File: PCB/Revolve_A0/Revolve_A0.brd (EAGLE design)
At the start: 100 x 100 mm, 409 parts, among them IC1 TMC2100-LA, IC12 TMC2100-LA, IC15 TMC2100-LA, IC2 TMC2100-LA, IC24 TMC2100-LA, IC29 LAN8710A, IC30 MTFC2GMDEA, IC31 CY7C65632, IC5 TMC2100-LA, IC6 74AHC1G126DCK, IC7 74AHC1G126DCK, Q1 AON6758, Q2 AON6758, Q3 AON6758, Q8 AON6758, U1 OSD3358-512M-BSM, U10 TPD4S012_DRY_6, U11 PCA9685PW, U19 CD4050BD, X1 22-05-7038-03, X10 22-05-7038-03, X11 22-05-7038-03, X12 22-05-7048-04, X13 22-05-7038-03, X14 22-05-7048-04, X15 22-05-7048-04, X16 22-05-7048-04, X17 22-05-7048-04, X18 22-05-7048-04, X19 22-05-7038-03, X2 MSTBA4, X20 MSTBA4, X21 MSTBA2, X22 22-05-7038-03, X24 HDMI, X25 22-05-7048-04, X26 MSTBA2, X29 22-05-7038-03, X3 MSTBA2, X4 22-05-7028-02, X5 22-05-7028-02, X6 22-05-7028-02, X7 22-05-7038-03, X8 22-05-7038-03, X9 22-05-7028-02, Y1 24MHz, Y3 25 MHz, Y4 12 MHz

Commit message: Working on the LAN layout
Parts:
- removed C106, C17, C19, C20, C22, C24, C27, C29, C31, C34, C43, C71: 0.1uF, rcl:C0402
- removed C116, C117, C118, C119, C120, C121, C122, C123, C124, C125, C126, C127, C128, C129, C130, C131: 47pF, rcl:C0402
- removed C139, C144, C145, C18, C21, C25, C36, C52, C62, C75, C76, C77, C78, C79, C81: 4.7uF, rcl:C0402
- removed C50: 10nF, rcl:C0402
- removed C90: 10uF, rcl:C0805
- removed C96: 100uF, Panasonic-EEEFK_EEEFP:RHS1V10MCN1GS
- removed IC1, IC12, IC15, IC2, IC24, IC5: TMC2100-LA, we-chip:QFN36-PAD
- removed IC31: CY7C65632, Revolve:QFN28
- removed R147: 0, DNI, rcl:R0402
- removed R148: 0, rcl:R0402
- removed R151: 10K, rcl:R0402
- removed R153: 22R, rcl:R0402
- removed R54, R86: 4.7K, rcl:R0402
- removed R91: 33, rcl:R0402
- removed U11: PCA9685PW, custom:SOP65P640X110-28N
- added C13: 0.1uF, rcl:C0402
- added C5: 18pF, rcl:C0402
- added H1, H2, H3, H4: MOUNT-HOLE3.2, holes:3,2
- added J1: (no value), OSD3358-SM-RED Platform:CTI-JTAG
- added Q9: MMBT2907, OSD3358-SM-RED Platform:SOT23-BEC
- added R143, R144: 4.7K, rcl:R0402
- added R26: 1M, rcl:R0402
- added SV3: (no value), con-lstb:MA04-2
- added SV4: (no value), con-lstb:MA03-1
- added SV5: (no value), con-lstb:MA04-1
- added U$13, U$14, U$15, U$16: TRINAMIC_TMC2130_QFN36, TMC2130-Eval_v13:TRINAMIC_QFN36
- added U2: TUSB2046BIRHBT, Texas Instruments_By_element14_Batch_1:QFN50P500X500X100-33N
- added U3, U4: TPD2E001DRSR, Texas Instruments_By_element14_Batch_1:SON95P315X315X80-7N
- added U5: SN74HC245DW, Texas Instruments_By_element14_Batch_1:SOIC127P1030X265-20N
- added U7: TLVH431, OSD3358-SM-RED Platform:SOT23-3
- added Y5: ABS07-32.768KHZ-T, OSD3358-SM-RED Platform:CRYSTAL_3.2X1.5
- C1: value 22nF -> 0.1uF
- C12, C138, C140, C141, C142: value 4.7uF -> 0.1uF
- C143: value 4.7uF -> 10uF
- C48, C80: value 10uF -> 22uF
- C6: value 0.1uF -> 18pF
- EEPROM_WP, PMIC_NRESET, SYS_5V, SYS_RTC_1V8, SYS_VDD1_3V3, SYS_VDD2_3V3, SYS_VDD3_3V3, VDDS_DDR, VDDS_PLL, VDD_CODE, VDD_MPU: value TPPAD1-13 -> TPB1,27; device testpad:P1-13 -> testpad:B1,27
- R1: value 0.1R -> 1.5K; device rcl:R0805 -> rcl:R0402
- R12: value 44.3K,1% -> 100K,1%
- R152: value 10K -> 10K,1%
- R2: value 0.1R -> 0,DNI; device rcl:R0805 -> rcl:R0402
- R22: value 10K,1% -> 13.3K,1%
- R24: value 4.7K -> 0R,DNI
- R41: value 10K -> 10K, 1%; device rcl:R0402 -> OSD3358-SM-RED Platform:R0402
- R49: value 10K -> 40.2K, 1%; device rcl:R0402 -> OSD3358-SM-RED Platform:R0402
- R53: value 2.2R -> 499; device rcl:R0402 -> OSD3358-SM-RED Platform:R0402
- R87: value 650R, 1% -> 4.7K
- SV2: device con-lstb:MA05-1 -> con-lstb:MA04-2
- U$9: value SN74AUC1G74DCTR -> TRINAMIC_TMC2130_QFN36; device Revolve:S-PDSO-G8 -> TMC2130-Eval_v13:TRINAMIC_QFN36
- Y1: value 24MHz -> 25MHz
- Y4: value 12 MHz -> 6 MHz
- moved PMIC_NRESET 474.8 mm to (44.7, 69.9), flipped to the bottom
- moved VDDS_PLL 452.8 mm to (38.5, 70.0), flipped to the bottom
- moved VDD_MPU 431.2 mm to (37.0, 70.0), flipped to the bottom
- moved VDD_CODE 397.7 mm to (38.8, 57.7), flipped to the bottom
- moved VDDS_DDR 376.0 mm to (37.3, 57.7), flipped to the bottom
- moved SV2 333.6 mm to (38.2, 33.5)
- moved EEPROM_WP 319.6 mm to (46.5, 51.6)
- moved R141 276.1 mm to (16.3, 23.8)
- moved R140 272.5 mm to (16.3, 24.9), turned to 180 degrees
- moved R138 255.3 mm to (20.8, 27.9), turned to 270 degrees
- moved R139 250.0 mm to (20.8, 16.6), turned to 90 degrees
- moved C88 240.6 mm to (16.3, 19.1), turned to 180 degrees
- moved C99 234.2 mm to (17.4, 17.2), turned to 270 degrees
- moved R126 232.9 mm to (16.3, 21.5)
- moved C87 232.5 mm to (16.3, 20.4), turned to 180 degrees
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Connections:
- net N$1 renamed PMIC_PWR_EN
- net N$103 renamed PMIC_SCL
- net N$104 renamed PMIC_SDA
- net N$121 renamed PMIC_LDO_PGOOD
- net N$143 renamed PMIC_NWAKEUP
- net N$144 renamed PMIC_NINT
- net N$157 renamed TXP
- net N$158 renamed TXN
- net N$159 renamed RXP
- net N$160 renamed RXN
- net N$174 renamed EEPROM_WP
- net VBUS renamed USB_HOST_5V
- removed net 12MHZ: R91.1, U$7.27
- removed net D+: U$8.P$3, U10.1
- removed net D-: U$8.P$2, U10.2
- removed net ENABLE_A: IC24.22
- removed net ENABLE_E: IC12.22
- removed net ENABLE_H: IC15.22
- removed net ENABLE_X: IC1.22, U$2.22
- removed net ENABLE_Y: IC2.22
- removed net ENABLE_Z: IC5.22
- removed net END_STOP_X_1: U19.2
- removed net END_STOP_X_2: U19.10
- removed net END_STOP_Y_1: U19.4
- removed net END_STOP_Y_2: U19.12
- removed net END_STOP_Z_1: U19.6
- removed net END_STOP_Z_2: U19.15
- removed net FAULT_X0: U$2.20
- removed net FAULT_X1: U$2.21
- removed net I2C2_SCL: U11.26
- removed net I2C2_SDA: U11.27
- removed net ID: U$8.P$4, U10.3
- removed net IREF_A_RAW: R73.2, U11.8
- removed net IREF_E_RAW: R60.2, U11.21
- removed net IREF_H1: C81.1, R43.2, R73.1
- removed net IREF_H_RAW: R31.2, U11.22
- removed net IREF_X1: C145.1, R140.2, R141.1
- removed net IREF_X_RAW: R141.2, R41.2, U11.18
- removed net IREF_Y_RAW: R37.2, U11.19
- removed net IREF_Z_RAW: R58.2, U11.20
- removed net N$100: IC15.5
- removed net N$101: IC15.18
- removed net N$102: IC15.19
- removed net N$105: SYS_VDD1_3V3.TP, U1.F6, U1.F7, U1.G6, U1.G7
- removed net N$107: C70.1, IC15.26, R52.2
- removed net N$108: C71.1, IC1.26, R53.2
- removed net N$110: C72.1, IC2.26, R59.2
- removed net N$111: C74.1, IC12.26, R71.2
- removed net N$112: IC12.32, X17.1
- removed net N$119: IC15.32, X18.1
- removed net N$120: SYS_VDD3_3V3.TP, U1.F8, U1.G8, U1.H7, U1.H8, U1.J7, U1.J8, U1.K8, U1.L8
- removed net N$131: C52.1, IC24.23, R43.1
- removed net N$133: IC24.3
- removed net N$135: IC24.34, X25.2
- removed net N$136: C55.2, IC24.25, R72.1
- removed net N$138: IC24.4
- removed net N$139: IC24.5
- removed net N$140: IC24.18
- removed net N$141: IC24.19
- removed net N$142: SYS_RTC_1V8.TP, U1.K11, U1.L11
- removed net N$146: U1.F9, U1.G9, U1.H9, U1.J9, U1.K9, U1.L9
- removed net N$148: IC24.32, X25.1
- removed net N$165: U1.T7
- removed net N$166: C86.2, R126.1, U$2.25
- removed net N$175: R86.2
- removed net N$178: U1.T16
- removed net N$18: IC1.14, R1.2
- removed net N$185: C144.1, R140.1, U$2.23
- removed net N$186: U1.T12
- removed net N$187: C155.1, IC31.27, R147.1, R148.1
- removed net N$188: U1.R12
- removed net N$190: U1.T13
- removed net N$191: IC31.14, IC31.21, IC31.28, IC31.5, IC31.9
- removed net N$197: IC31.13, U$6.3
- removed net N$198: IC31.12, U$6.2
- removed net N$199: IC31.16, U$6.7
- removed net N$200: IC31.15, U$6.6
- removed net N$202: U$9.2, U$9.3
- removed net N$205: R91.2, U$9.5
- removed net N$210: SV2.5, U1.B12
- removed net N$213: C157.2, IC31.11, Y4.P$1
- removed net N$215: SV2.4, U1.A12
- removed net N$26: C25.1, IC5.23, R27.1
- removed net N$31: C21.2, IC1.25, R53.1
- removed net N$47: C33.2, IC2.25, R59.1
- removed net N$50: IC5.34, X16.2
- removed net N$51: C37.2, IC5.25, R70.1
- removed net N$53: IC2.5
- removed net N$54: IC5.4
- removed net N$55: IC5.5
- removed net N$56: IC2.18
- removed net N$57: IC5.18
- removed net N$58: IC5.19
- removed net N$60: C50.2, L1.P$2, U$10.2
- removed net N$65: IC2.19
- removed net N$73: C50.1, U$10.6
- removed net N$74: C62.1, IC12.23, R35.1
- removed net N$76: IC12.3
- removed net N$78: IC12.34, X17.2
- removed net N$79: C65.2, IC12.25, R71.1
- removed net N$81: IC12.4
- removed net N$82: IC12.5
- removed net N$83: IC12.18
- removed net N$84: IC12.19
- removed net N$89: C36.1, IC15.23, R50.1
- removed net N$91: IC15.3
- removed net N$94: IC15.34, X18.2
- removed net N$95: C68.2, IC15.25, R52.1
- removed net N$99: IC15.4
- removed net SPI0_CS0: U1.A14
- removed net SPI0_CS1: U1.C14
- removed net USB1_OCN: U1.R15
- removed net XDMA_EVENT_INTR0: U$9.1, U1.A4
- removed net X_CFG1: IC1.4
- removed net X_CFG2: IC1.3
- new net 5VIN_Y: C72.1, R59.2, U$13.26
- new net 5VOUT_A: C55.2, R72.1, R73.2, U$16.25
- new net 5VOUT_E: C65.2, R35.2, R71.1, U$14.25
- new net 5VOUT_H: C68.2, R31.2, R52.1, U$15.25
- new net 5VOUT_X: C86.2, R126.1, R140.2, U$2.25
- new net 5VOUT_Y: C33.2, R37.2, R59.1, U$13.25
- new net 5VOUT_Z: C37.2, R27.2, R70.1, U$9.25
- new net CLKOUT1_25MHZ: R2.1, U1.A4
- new net CLKOUT2_48MHZ: U1.B4, U2.27
- new net ECAP1: SV5.3, U1.B12
- new net ECAP2: SV5.2, U1.A12
- new net EHRPWM1A: U1.P12, U5.6
- new net EHRPWM1B: U1.T13, U5.7
- new net EHRPWM2A: U1.T4, U5.8
- new net EHRPWM2B: U1.P5, U5.9
- new net EMU0: J1.13, U1.E2
- new net EMU1: J1.14, U1.E3
- new net ENABLE_B: SV2.4
- new net ENABLE_C: SV3.3
- new net END_STOP_X1: U1.N14, U19.2
- new net END_STOP_X2: U1.R12, U19.10
- new net END_STOP_Y1: U1.T16, U19.4
- new net END_STOP_Y2: U1.P3, U19.12
- new net END_STOP_Z1: U1.T6, U19.6
- new net END_STOP_Z2: U1.P7, U19.15
- new net FAULT_A: R44.1, U$16.20, U$16.21
- new net FAULT_B: SV2.2
- new net FAULT_C: SV3.1
- new net GPIO0_18: U1.J15
- new net GPIO0_26: U1.R5
- new net I2C1_SCL: U1.B11
- new net I2C1_SDA: U1.A11
- new net N$1: R41.1, R49.2, U7.1
- new net N$25: R152.1, U1.M16
- new net QUAD_ENCODER_A: U1.R13
- new net QUAD_ENCODER_B: U1.P13
- new net SPI0_CSA: U$16.2, U1.J14
- new net SPI0_CSE: U$14.2, U1.T12
- new net SPI0_CSH: U$15.2, U1.R7
- new net SPI0_CSY: U$13.2, U1.C14
- new net SPI0_CSZ: U$9.2, U1.T7
- new net SPI1_CS0: SV3.4, U1.B10
- new net SPI1_CS1: SV2.3, U1.A10
- new net SPI1_MISO: SV2.6, SV3.6, U1.C12
- new net SPI1_MOSI: SV2.8, SV3.8, U1.C13
- new net SPI1_SCLK: SV2.1, SV3.2, U1.C5
- new net SW: C2.1, L1.P$2, U$10.2
- new net SYS_RTC_1V8: Q9.C, R49.1, SYS_RTC_1V8.TP, U1.K11, U1.L11, U7.3
- new net SYS_VDD1_3V3: C13.1, C140.1, C141.1, C142.1, C143.1, C150.1, C155.1, IC29.12, IC30.C6, IC30.E6, IC30.F5, IC30.J10, IC30.K9, IC30.M4, IC30.N4, IC30.P3, IC30.P5, L2.1, R1.2, R127.2, R128.2, R129.2, R130.2, R131.2, R132.2, R133.2, R134.2, R135.2, R136.2, R137.2, R24.1, R85.1, R88.2, SYS_VDD1_3V3.TP, U1.F6, U1.F7, U1.G6, U1.G7, U2.25, U2.26, U2.3
- new net SYS_VDD3_3V3: Q9.E, R41.2, R53.2, SYS_VDD3_3V3.TP, U1.F8, U1.F9, U1.G8, U1.G9, U1.H7, U1.H8, U1.H9, U1.J7, U1.J8, U1.J9, U1.K8, U1.K9, U1.L8, U1.L9
- new net TCK: J1.11, U1.D1
- new net TDI: J1.3, U1.C1
- new net TDO: J1.7, U1.C2
- new net TIMER4: U1.M1, U5.2
- new net TIMER5: U1.N3, U5.3
- new net TIMER6: U1.N2, U5.4
- new net TIMER7: U1.N1, U5.5
- new net TK_A: U1.D7
- new net TK_E: U1.C7
- new net TK_H: U1.C8
- new net TK_HBP: U1.C9
- new net TMS: J1.1, U1.D2
- new net TRSRTN: J1.2
- new net TRSTN: U1.D3
- new net UART4_RXD: SV4.1, U1.P15
- new net UART4_TXD: SV4.2, U1.R16
- new net USB1_DM3: U$6.2, U2.19, U4.3
- new net USB1_DM4: U$6.6, U2.23, U3.3
- new net USB1_DP3: U$6.3, U2.20, U4.6
- new net USB1_DP4: U$6.7, U2.24, U3.6
- new net USB_XTAL1: C157.2, U2.30, Y4.P$1
- new net VCC: U3.1, U4.1
- new net VCC_E: C74.1, R71.2, U$14.26
- new net VCC_H: C70.1, R52.2, U$15.26
- net +24V: now also C1.2, U$13.16, U$13.30, U$13.31, U$14.16, U$14.30, U$14.31, U$15.16, U$15.30, U$15.31, U$16.16, U$16.30, U$16.31, U$9.16, U$9.30, U$9.31; no longer C19.1, C20.2, C22.2, C24.1, C27.1, C29.1, C31.1, C34.1, C43.1, C6.1, C90.1, C96.+, IC1.16, IC1.30, IC1.31, IC12.16, IC12.30, IC12.31, IC15.16, IC15.30, IC15.31, IC2.16, IC2.30, IC2.31, IC24.16, IC24.30, IC24.31, IC5.16, IC5.30, IC5.31
- net +3V3: now also R143.1, R144.1, U$13.8, U$14.8, U$15.8, U$16.8; no longer C106.1, C2.1, IC1.8, IC12.8, IC15.8, IC2.8, IC24.8, IC5.8, R24.2, R54.2, U$9.6, U$9.7
- net +5V: no longer R147.2
- net CGND: now also U$3.SHD1, U$3.SHD2, U$5.A10, U$5.A11, U$5.A12, U$5.A9, U$6.A10, U$6.A11, U$6.A12, U$6.A9, U$8.P$10, U$8.P$11, U$8.P$6, U$8.P$7, U$8.P$8, U$8.P$9, X24.PAD1, X24.PAD2, X24.PAD3, X24.PAD4
- net DIR_A: now also U$16.7; no longer IC24.7
- net DIR_B: now also SV2.5
- net DIR_C: now also SV3.5
- net DIR_E: now also U$14.7; no longer IC12.7
- net DIR_H: now also U$15.7; no longer IC15.7
- net DIR_X: no longer IC1.7
- net DIR_Y: now also U$13.7; no longer IC2.7
- net DIR_Z: now also U$9.7; no longer IC5.7
- net EMMC_RST: no longer U1.R13
- net ENABLE: now also U5.19; no longer U11.23
- net FAN0: now also U5.14; no longer U11.13
- net FAN1: now also U5.13; no longer U11.15
- net FAN2: now also U5.12; no longer U11.16
- net FAN3: now also U5.11; no longer U11.17
- net FAULT_E: now also U$14.20, U$14.21; no longer IC12.20
- net FAULT_H: now also U$15.20, U$15.21; no longer IC15.20, IC24.20, R44.1
- net FAULT_X: now also R143.2, U$2.20, U$2.21, U1.T5; no longer IC1.20, R54.1
- net FAULT_Y: now also R144.2, U$13.20, U$13.21; no longer IC2.20, R24.1
- net FAULT_Z: now also U$9.20, U$9.21; no longer IC5.20
- net GND: now also C1.1, C13.2, J1.10, J1.12, J1.16, J1.20, J1.8, R141.1, R152.2, R43.1, R50.1, R58.1, R6.1, R60.1, SV4.3, SV5.1, U$13.1, U$13.11, U$13.12, U$13.17, U$13.22, U$13.24, U$13.35, U$13.36, U$13.9, U$13.GND_PAD, U$14.1, U$14.11, U$14.12, U$14.17, U$14.22, U$14.24, U$14.35, U$14.36, U$14.9, U$14.GND_PAD, U$15.1, U$15.11, U$15.12, U$15.17, U$15.22, U$15.24, U$15.35, U$15.36, U$15.9, U$15.GND_PAD, U$16.1, U$16.11, U$16.12, U$16.17, U$16.22, U$16.24, U$16.35, U$16.36, U$16.9, U$16.GND_PAD, U$2.22, U$2.9, U$9.1, U$9.11, U$9.12, U$9.17, U$9.22, U$9.24, U$9.35, U$9.36, U$9.9, U$9.GND_PAD, U2.28, U2.7, U2.8, U5.10; no longer C106.2, C116.2, C117.2, C118.2, C119.2, C120.2, C121.2, C122.2, C123.2, C124.2, C125.2, C126.2, C127.2, C128.2, C129.2, C130.2, C131.2, C139.2, C144.2, C145.2, C17.2, C18.2, C19.2, C2.2, C20.1, C21.1, C24.2, C25.2, C27.2, C29.2, C31.2, C34.2, C36.2, C43.2, C52.2, C6.2, C62.2, C71.2, C75.2, C76.2, C77.2, C78.2, C79.2, C81.2, C90.2, C96.-, IC1.1, IC1.10, IC1.11, IC1.12, IC1.24, IC1.35, IC1.36, IC1.TP, IC12.1, IC12.10, IC12.11, IC12.12, IC12.24, IC12.35, IC12.36, IC12.TP, IC15.1, IC15.10, IC15.11, IC15.12, IC15.24, IC15.35, IC15.36, IC15.TP, IC2.1, IC2.10, IC2.11, IC2.12, IC2.24, IC2.35, IC2.36, IC2.TP, IC24.1, IC24.10, IC24.11, IC24.12, IC24.24, IC24.35, IC24.36, IC24.TP, IC31.29, IC5.1, IC5.10, IC5.11, IC5.12, IC5.24, IC5.35, IC5.36, IC5.TP, R1.1, R151.1, R2.1, R86.1, SV2.1, U$5.A10, U$5.A11, U$5.A12, U$5.A9, U$6.A10, U$6.A11, U$6.A12, U$6.A9, U$8.P$10, U$8.P$11, U$8.P$6, U$8.P$7, U$8.P$8, U$8.P$9, U$9.4, U11.14
- net HDMI_1V8: now also C12.1
- net HDMI_INT: now also U1.R15; no longer U1.T15
- net HEATER_A: now also U5.15; no longer U11.12
- net HEATER_E: now also U5.18; no longer U1.P12
- net HEATER_H: now also U5.17; no longer U11.9
- net HEATER_HBP: now also U5.16; no longer U11.10
- net IREF_E: now also R35.1, R60.2, U$14.23; no longer C79.1, R35.2, R60.1
- net IREF_H: now also U$15.23; no longer C75.1
- net IREF_X: now also R140.1, R141.2, U$2.23; no longer C77.1, R41.1, R49.2
- net IREF_Y: now also U$13.23; no longer C76.1
- net IREF_Z: now also R27.1, R58.2, U$9.23; no longer C78.1, R27.2, R58.1
- net LCD_D0: no longer C116.1
- net LCD_D1: no longer C117.1
- net LCD_D10: no longer C126.1
- net LCD_D11: no longer C127.1
- net LCD_D12: no longer C128.1
- net LCD_D13: no longer C129.1
- net LCD_D14: no longer C130.1
- net LCD_D15: no longer C131.1
- net LCD_D2: no longer C118.1
- net LCD_D3: no longer C119.1
- net LCD_D4: no longer C120.1
- net LCD_D5: no longer C121.1
- net LCD_D6: no longer C122.1
- net LCD_D7: no longer C123.1
- net LCD_D8: no longer C124.1
- net LCD_D9: no longer C125.1
- net LCD_DE: no longer R153.2
- net LCD_PCLK: no longer R153.1
- net N$109: now also U$9.26; no longer IC5.26
- net N$113: now also U$15.13; no longer IC15.13
- net N$12: now also U$15.27; no longer IC15.27
- net N$126: now also U$16.14; no longer IC24.14
- net N$128: now also U$16.33; no longer IC24.33
- net N$13: now also U$15.14; no longer IC15.14
- net N$132: now also U$16.28; no longer IC24.28
- net N$134: now also U$16.15; no longer IC24.15
- net N$137: now also U$16.29; no longer IC24.29
- net N$14: now also U$9.27; no longer IC5.27
- net N$145: now also U$16.26; no longer IC24.26
- net N$147: now also U$16.13; no longer IC24.13
- net N$15: now also U$9.14; no longer IC5.14
- net N$16: now also U$9.32, X16.2; no longer C1.1, IC1.28
- net N$17: now also U2.10, U2.14, U2.18, U2.22; no longer C1.2, IC1.27
- net N$180: now also R2.2
- net N$19: now also U$13.32, X15.2; no longer IC1.33, R2.2
- net N$192: now also R24.2, U2.31; no longer IC31.8
- net N$193: now also U2.12; no longer IC31.4
- net N$194: now also U2.11; no longer IC31.3
- net N$195: now also U2.16; no longer IC31.7
- net N$196: now also U2.15; no longer IC31.6
- net N$2: now also U$13.13; no longer IC2.13
- net N$20: now also U$13.34, X15.1; no longer C12.1, IC1.23, R49.1
- net N$214: now also U2.29; no longer IC31.10
- net N$22: now also U$14.34, X17.1; no longer IC2.32, X15.1
- net N$24: now also U$9.33; no longer IC5.33
- net N$27: now also U$9.28; no longer IC5.28
- net N$28: now also U$14.32, X17.2; no longer IC5.3
- net N$29: now also U$9.15; no longer IC5.15
- net N$3: now also U$13.27; no longer IC2.27
- net N$30: now also U$15.33; no longer IC15.33
- net N$32: now also U$15.34, X18.1; no longer IC5.32, X16.1
- net N$33: now also C5.1, C6.1, U1.B5; no longer C22.1, IC1.29
- net N$35: now also U$13.14; no longer IC2.14
- net N$36: now also U$13.33; no longer IC2.33
- net N$37: now also U$9.13; no longer IC5.13
- net N$38: now also U$15.32, X18.2; no longer C18.1, IC2.23, R6.1
- net N$39: now also U$14.13; no longer IC12.13
- net N$4: now also Q9.B, R53.1, U7.2; no longer SV2.3, U1.C12
- net N$41: now also U$13.28; no longer IC2.28
- net N$42: now also C6.2, R26.2, U1.A5, Y5.P$2; no longer IC2.3
- net N$43: now also C5.2, R26.1, U1.A6, Y5.P$1; no longer IC1.19
- net N$44: now also U$16.34, X25.1; no longer IC1.5
- net N$45: now also U$13.15; no longer IC2.15
- net N$46: now also U$16.32, X25.2; no longer IC2.34, X15.2
- net N$48: now also U$13.29; no longer IC2.29
- net N$49: now also R43.2, R73.1, U$16.23; no longer IC2.4
- net N$5: now also C2.2, U$10.6; no longer SV2.2, U1.C13
- net N$52: now also U$9.29; no longer IC5.29
- net N$6: now also U$9.34, X16.1; no longer IC1.18
- net N$70: now also U$14.27; no longer IC12.27
- net N$71: now also U$14.14; no longer IC12.14
- net N$72: now also U$14.33; no longer IC12.33
- net N$75: now also U$14.28; no longer IC12.28
- net N$77: now also U$14.15; no longer IC12.15
- net N$80: now also U$14.29; no longer IC12.29
- net N$90: now also U$15.28; no longer IC15.28
- net N$92: now also U$15.15; no longer IC15.15
- net N$96: now also U$16.27; no longer IC24.27
- net N$98: now also U$15.29; no longer IC15.29
- net SPI0_CSX: now also U1.A14
- net SPI0_MISO: now also U$13.5, U$14.5, U$15.5, U$16.5, U$9.5
- net SPI0_MOSI: now also U$13.4, U$14.4, U$15.4, U$16.4, U$9.4
- net SPI0_SCLK: now also U$13.3, U$14.3, U$15.3, U$16.3, U$9.3
- net STEP_A: now also U$16.6; no longer IC24.6
- net STEP_B: now also SV2.7
- net STEP_C: now also SV3.7
- net STEP_E: now also U$14.6; no longer IC12.6
- net STEP_H: now also U$15.6; no longer IC15.6
- net STEP_X: no longer IC1.6
- net STEP_Y: now also U$13.6; no longer IC2.6
- net STEP_Z: now also U$9.6; no longer IC5.6
- net SYS_5V: now also U5.1, U5.20; no longer C17.1, R148.2, R88.2, U11.1, U11.2, U11.24, U11.28, U11.3, U11.4, U11.5
- net SYS_RESETN: now also U1.N12, U1.P11, U1.R11
- net SYS_VDD2_3V3: now also SV5.4
- net USB0_DM: now also U$8.P$2, U10.2
- net USB0_DP: now also U$8.P$3, U10.1
- net USB0_ID: now also U$8.P$4, U10.3
- net USB1_DM: now also U2.2; no longer IC31.1
- net USB1_DP: now also R1.1, U2.1; no longer IC31.2
- net USB_DC: no longer IC31.22, R151.2
- net USB_RESET: now also U2.4; no longer IC31.17
- net USR0: now also U1.T15; no longer U1.P13
- net VDD_3V3B: no longer C139.1, C140.1, C141.1, C142.1, C143.1, C150.1, IC29.12, IC30.C6, IC30.E6, IC30.F5, IC30.J10, IC30.K9, IC30.M4, IC30.N4, IC30.P3, IC30.P5, L2.1, R127.2, R128.2, R129.2, R130.2, R131.2, R132.2, R133.2, R134.2, R135.2, R136.2, R137.2, R85.1
- net X_A1: now also X14.1; no longer X14.2
- net X_A2: now also X14.2; no longer X14.1
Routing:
- net SPI0_MISO: track 0.00 -> 164.0 mm, vias 0 -> 7
- net FAN3: track 148.3 -> 0.00 mm, vias 2 -> 0
- net FAN2: track 141.6 -> 0.00 mm, vias 2 -> 0
- net FAN1: track 136.2 -> 0.00 mm, vias 2 -> 0
- net FAN0: track 135.4 -> 0.00 mm, vias 4 -> 0
- net SYS_RESETN: track 12.6 -> 141.1 mm, vias 0 -> 5
- net SPI0_MOSI: track 0.00 -> 125.8 mm, vias 0 -> 6
- net SPI0_SCLK: track 0.00 -> 121.9 mm, vias 0 -> 6
- net IREF_A_RAW: track 113.0 -> 0.00 mm, vias 4 -> 0
- net SYS_5V: track 94.9 -> 0.64 mm, vias 4 -> 1
- net IREF_H_RAW: track 82.0 -> 0.00 mm, vias 2 -> 0
- net N$125: track 1.12 -> 76.7 mm, vias 0 -> 2
- net N$124: track 1.18 -> 75.7 mm, vias 0 -> 2
- net N$123: track 1.18 -> 74.7 mm, vias 0 -> 2
- net N$201: track 0.00 -> 73.0 mm, vias 0 -> 2
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- added copper zone on layer 1, net +5V
- added copper zone on layer 3, net N$18
- added copper zone on layer 1, net SW
- added copper zone on layer 3, net SW
- added copper zone on layer 1, net SYS_5V
- added copper zone on layer 1, net SYS_RTC_1V8
- added copper zone on layer 1, net SYS_VDD1_3V3
- added copper zone on layer 3, net SYS_VDD1_3V3
- added copper zone on layer 1, net SYS_VDD2_3V3
- added copper zone on layer 1, net SYS_VDD3_3V3
- added copper zone on layer 1, net SYS_VDD_1V8
- added copper zone on layer 1, net USB_DC
- added copper zone on layer 1, net VIN_BAT
- removed copper zone on layer 3, net VDD_3V3B
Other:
- outline, holes or cut-outs redrawn

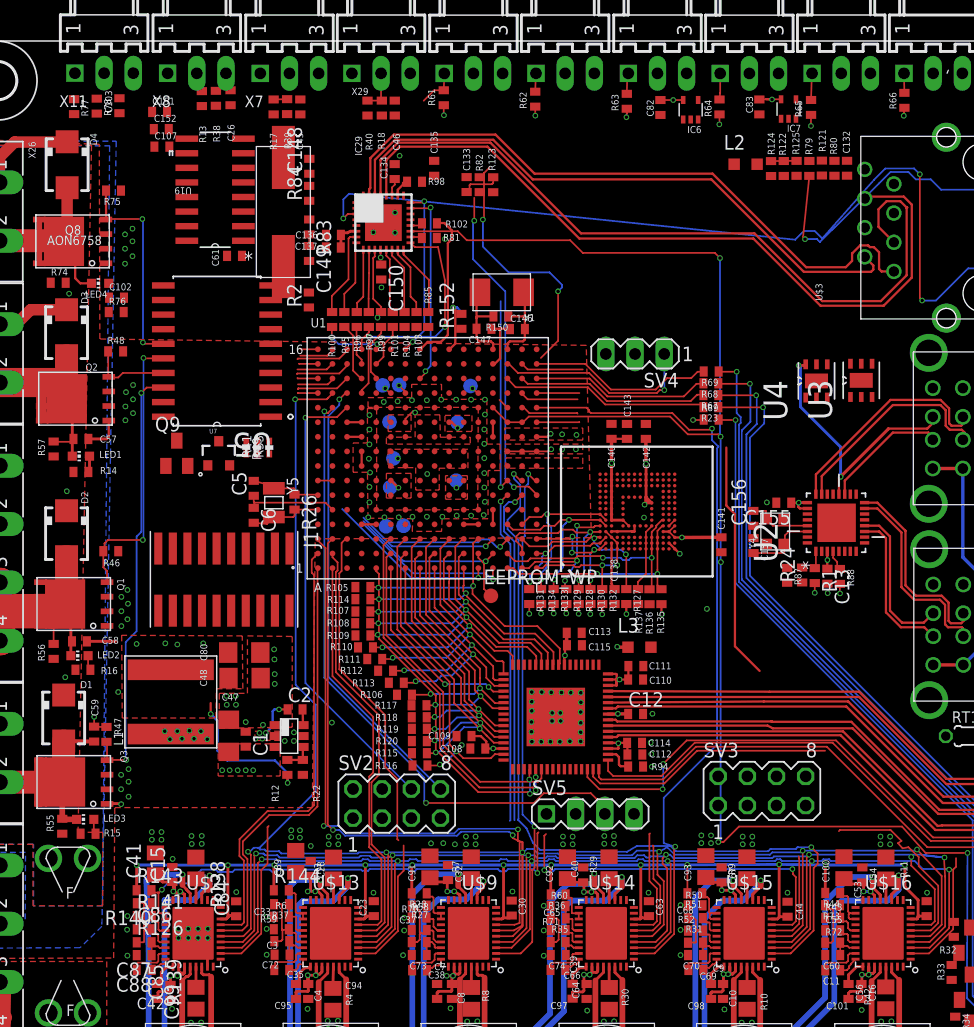
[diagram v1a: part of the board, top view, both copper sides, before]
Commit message: Working on layout
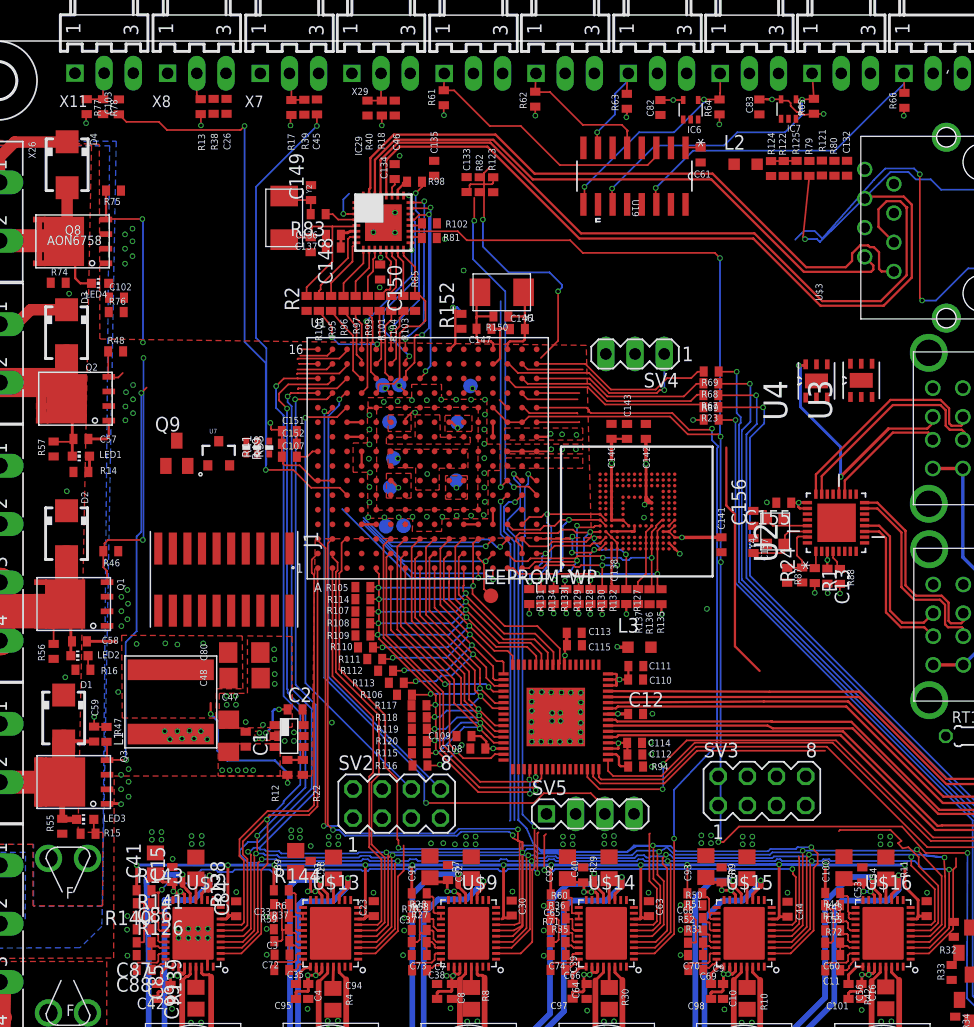
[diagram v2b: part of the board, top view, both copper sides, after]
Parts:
- removed C5, C6: 18pF, rcl:C0402
- removed R26, R84: 1M, rcl:R0402
- removed U5: SN74HC245DW, Texas Instruments_By_element14_Batch_1:SOIC127P1030X265-20N
- removed Y3: 25 MHz, Revolve:ECS-250-20-5PVX
- removed Y5: ABS07-32.768KHZ-T, OSD3358-SM-RED Platform:CRYSTAL_3.2X1.5
- added Y2: 25MHz, Revolve:445C33D24M00000
- moved C61 41.5 mm to (64.7, 90.0), turned to 270 degrees
- moved U19 36.5 mm to (59.0, 88.2), turned to 270 degrees
- moved C151 30.0 mm to (28.9, 66.0)
- moved C152 29.6 mm to (28.9, 64.9)
- moved C107 29.2 mm to (28.9, 63.8)
- moved C148 6.83 mm to (30.8, 82.2), turned to 270 degrees
- moved C149 5.30 mm to (30.8, 86.8), turned to 90 degrees
- moved R95 1.81 mm to (32.5, 77.1)
- moved R96 1.81 mm to (33.6, 77.1)
- moved R100 1.81 mm to (31.5, 77.1)
- moved R101 1.81 mm to (36.8, 77.1)
- moved R103 1.81 mm to (38.8, 77.1)
- moved R104 1.81 mm to (37.8, 77.1)
- moved R85 1.81 mm to (39.8, 77.1)
- moved R97 1.81 mm to (34.7, 77.1)
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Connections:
- removed net +3V3: C23.1, C30.1, C44.1, C53.1, C61.1, C63.1, C84.1, R114.2, R117.2, R118.2, R119.2, R120.2, R143.1, R144.1, R28.2, R36.2, R44.2, R51.2, U$13.8, U$14.8, U$15.8, U$16.8, U$2.8, U$9.8, U19.1
- removed net ENABLE: U5.19
- removed net N$33: C5.1, C6.1, U1.B5
- removed net N$42: C6.2, R26.2, U1.A5, Y5.P$2
- removed net N$43: C5.2, R26.1, U1.A6, Y5.P$1
- net EHRPWM1A: no longer U5.6
- net EHRPWM1B: no longer U5.7
- net EHRPWM2A: no longer U5.8
- net EHRPWM2B: no longer U5.9
- net FAN0: no longer U5.14
- net FAN1: no longer U5.13
- net FAN2: no longer U5.12
- net FAN3: no longer U5.11
- net GND: now also X11.3, X7.3, X8.3; no longer U5.10
- net HEATER_A: no longer U5.15
- net HEATER_E: no longer U5.18
- net HEATER_H: no longer U5.17
- net HEATER_HBP: no longer U5.16
- net N$151: now also X11.2
- net N$180: now also Y2.P$2; no longer R84.2, Y3.P$2
- net N$181: now also Y2.P$1; no longer Y3.P$1
- net N$183: no longer R84.1
- net N$237: now also X8.2
- net N$241: now also X7.2
- net SYS_5V: no longer U5.1, U5.20
- net SYS_VDD1_3V3: now also C23.1, C30.1, C44.1, C53.1, C61.1, C63.1, C84.1, R114.2, R117.2, R118.2, R119.2, R120.2, R143.1, R144.1, R28.2, R36.2, R44.2, R51.2, U$13.8, U$14.8, U$15.8, U$16.8, U$2.8, U$9.8, U19.1
- net TIMER4: no longer U5.2
- net TIMER5: no longer U5.3
- net TIMER6: no longer U5.4
- net TIMER7: no longer U5.5
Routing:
- net SYS_VDD1_3V3: track 41.1 -> 160.0 mm, vias 19 -> 31
- net +3V3: track 118.3 -> 0.00 mm, vias 12 -> 0
- net TERM_A: track 0.00 -> 51.7 mm, vias 0 -> 2
- net SPI0_SCLK: track 121.9 -> 169.1 mm, vias 6 -> 7
- net SPI0_MOSI: track 125.8 -> 170.6 mm, vias 6 -> 8
- net SPI0_CSX: track 15.7 -> 58.2 mm, vias 0 -> 2
- net N$155: track 80.5 -> 40.9 mm
- net TERM_HBP: track 0.00 -> 33.1 mm, vias 0 -> 1
- net END_STOP_Z_2_IN: track 2.31 -> 30.1 mm, vias 0 -> 1
- net END_STOP_Y_2_IN: track 2.94 -> 26.9 mm, vias 0 -> 2
- net STEP_E: track 38.3 -> 61.8 mm, vias 0 -> 2
- net END_STOP_X_1_IN: track 3.59 -> 23.7 mm
- net MII1_TXD3: track 0.00 -> 17.6 mm, vias 0 -> 2
- net MII1_TXEN: track 0.00 -> 17.2 mm, vias 0 -> 2
- net END_STOP_X_2_IN: track 2.27 -> 19.4 mm, vias 0 -> 2
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- added copper zone on layer 3, net VDD_ADC
- removed copper zone on layer 3, net +3V3
